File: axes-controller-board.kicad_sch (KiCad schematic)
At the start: 62 parts, among them IC1 TPS5450QDDARQ1, J10 Conn_01x08, J11 Conn_01x04, J12 Conn_01x08, J13 Conn_01x04, J14 Conn_01x08, J15 Conn_01x08, J16 Conn_01x04, J17 Conn_01x08, J18 Conn_01x08, J19 Conn_01x04, J2 Conn_01x03, J20 Conn_01x08, J21 Conn_01x08, J22 Conn_01x04, J23 Conn_01x08, J24 Conn_01x08, J25 Conn_01x04, J26 Conn_01x08, J27 Raspberry_Pi_2_3, J28 DC1, J29 DC2, J3 Conn_01x03, J30 DC3, J31 Conn_01x08, J32 Conn_01x08, J33 DC1, J34 Conn_01x08, J35 Conn_01x08, J36 Conn_01x08, J4 Conn_01x03, J5 DRIVER, J6 NTC, J7 DRIVER, J8 NTC, J9 Conn_01x08, U1 LM1117MP-3.3

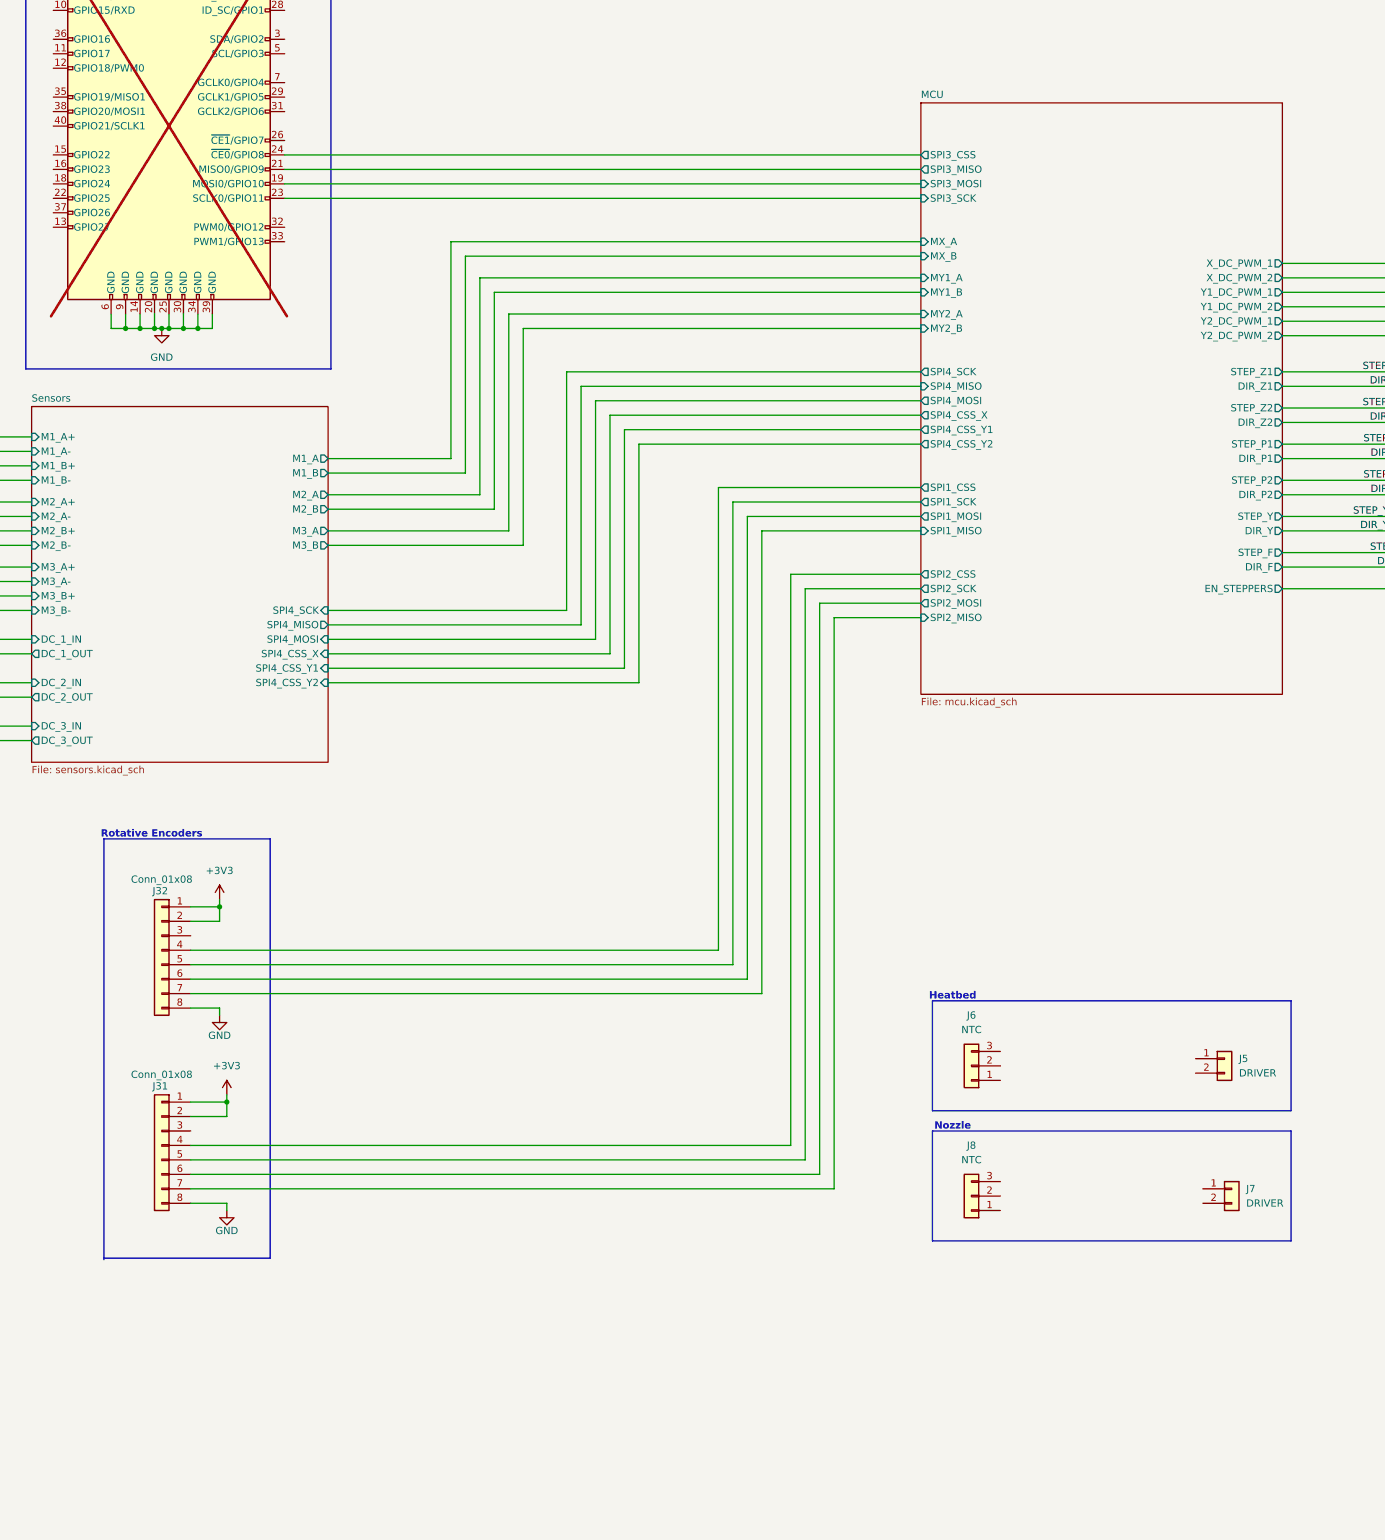
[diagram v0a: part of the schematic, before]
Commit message: feat: endstops integration
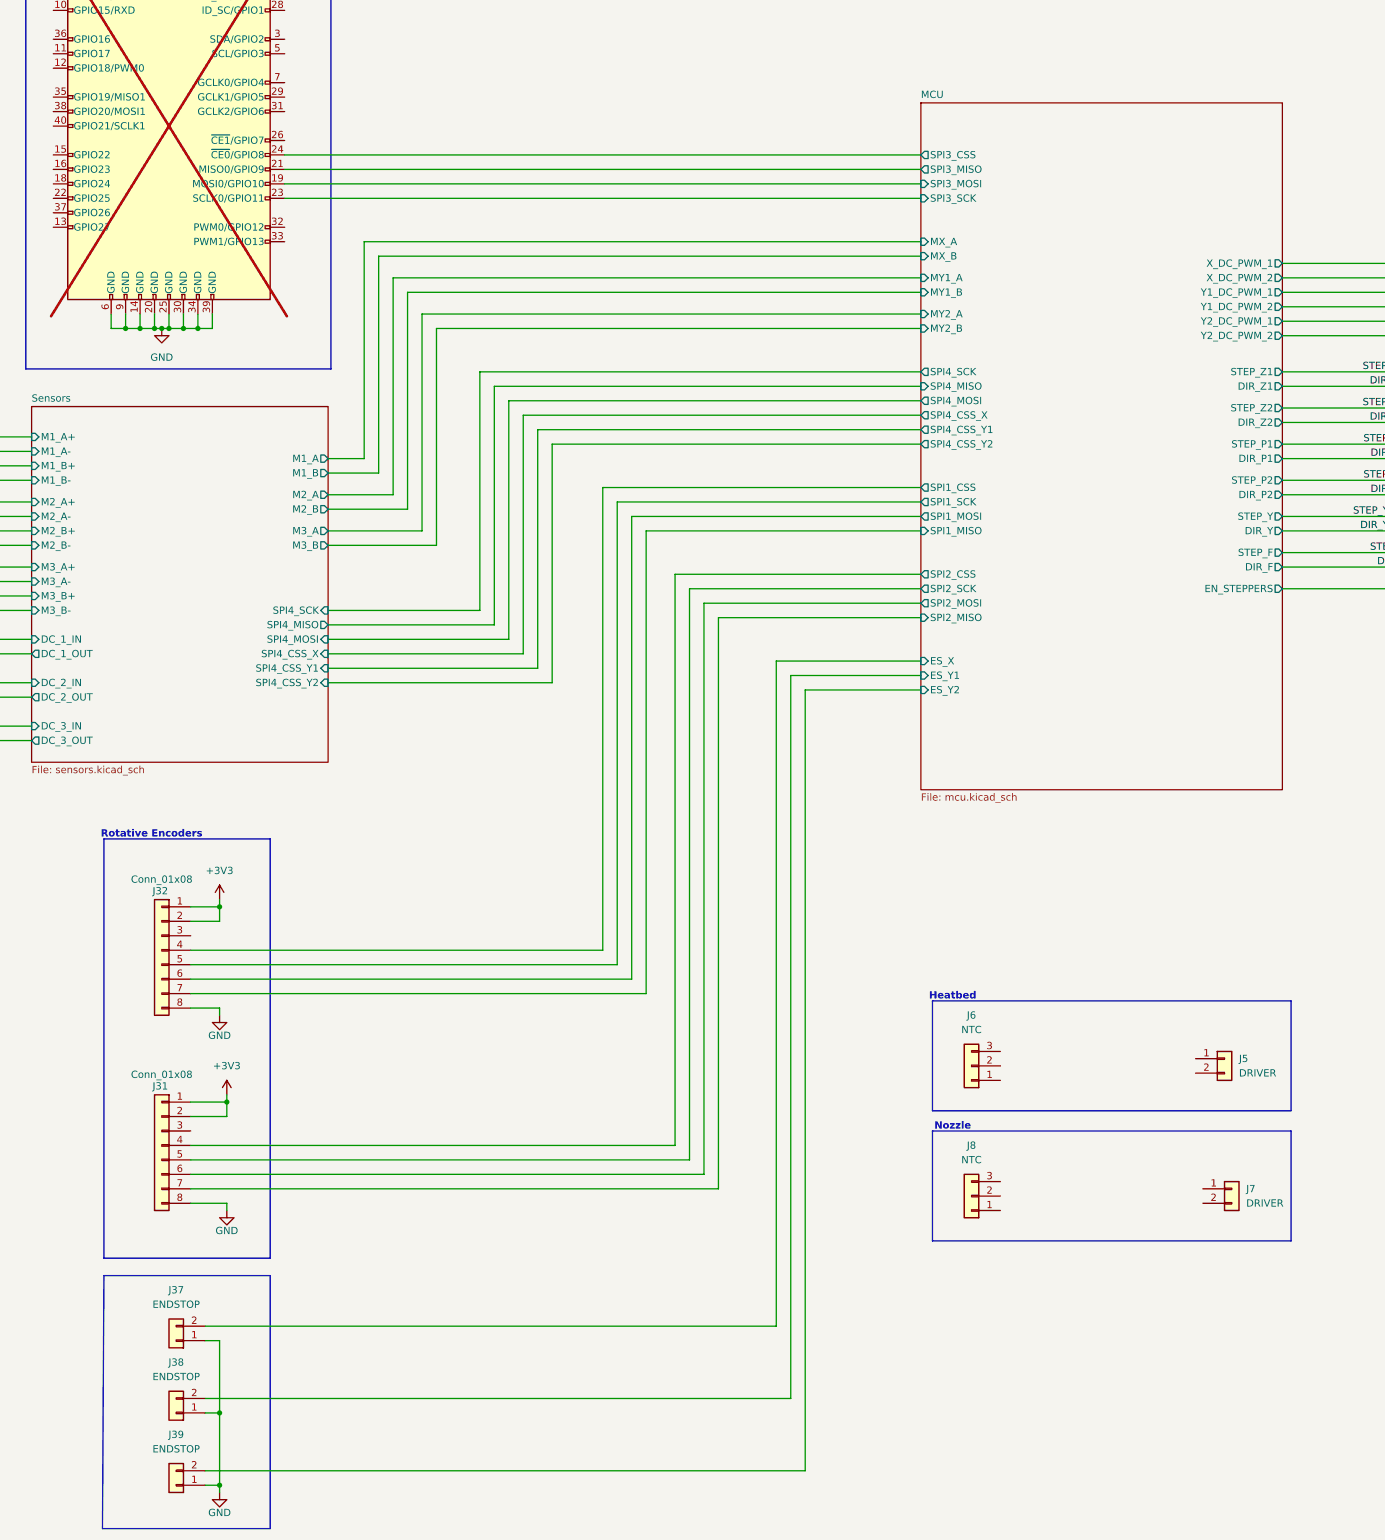
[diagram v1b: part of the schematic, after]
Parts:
- added J37, J38, J39: ENDSTOP, Connector_PinHeader_2.54mm:PinHeader_1x02_P2.54mm_Vertical, symbol Connector_Generic:Conn_01x02
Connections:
- net GND: now also J37.1 (Pin_1), J38.1 (Pin_1), J39.1 (Pin_1)
- new net MCU/ES_X: J37.2 (Pin_2)
- new net MCU/ES_Y1: J38.2 (Pin_2)
- new net MCU/ES_Y2: J39.2 (Pin_2)
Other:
- sheet MCU ports: added ES_X, ES_Y1, ES_Y2; removed none
